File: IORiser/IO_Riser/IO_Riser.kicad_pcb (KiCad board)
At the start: 2 copper layers, 29.9 x 82.4 mm, 4 parts, among them J1 I/O Port, J2 I/O Port

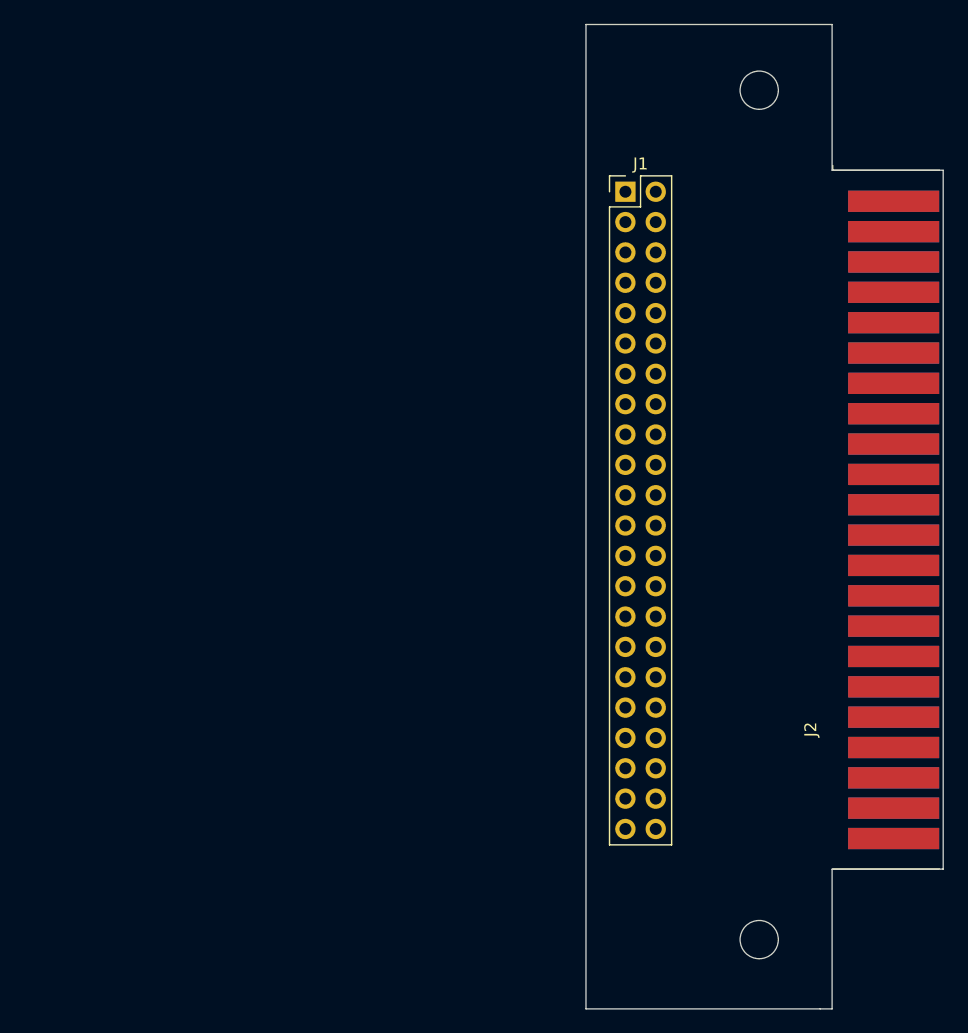
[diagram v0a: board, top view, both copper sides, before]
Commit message: PCB updates
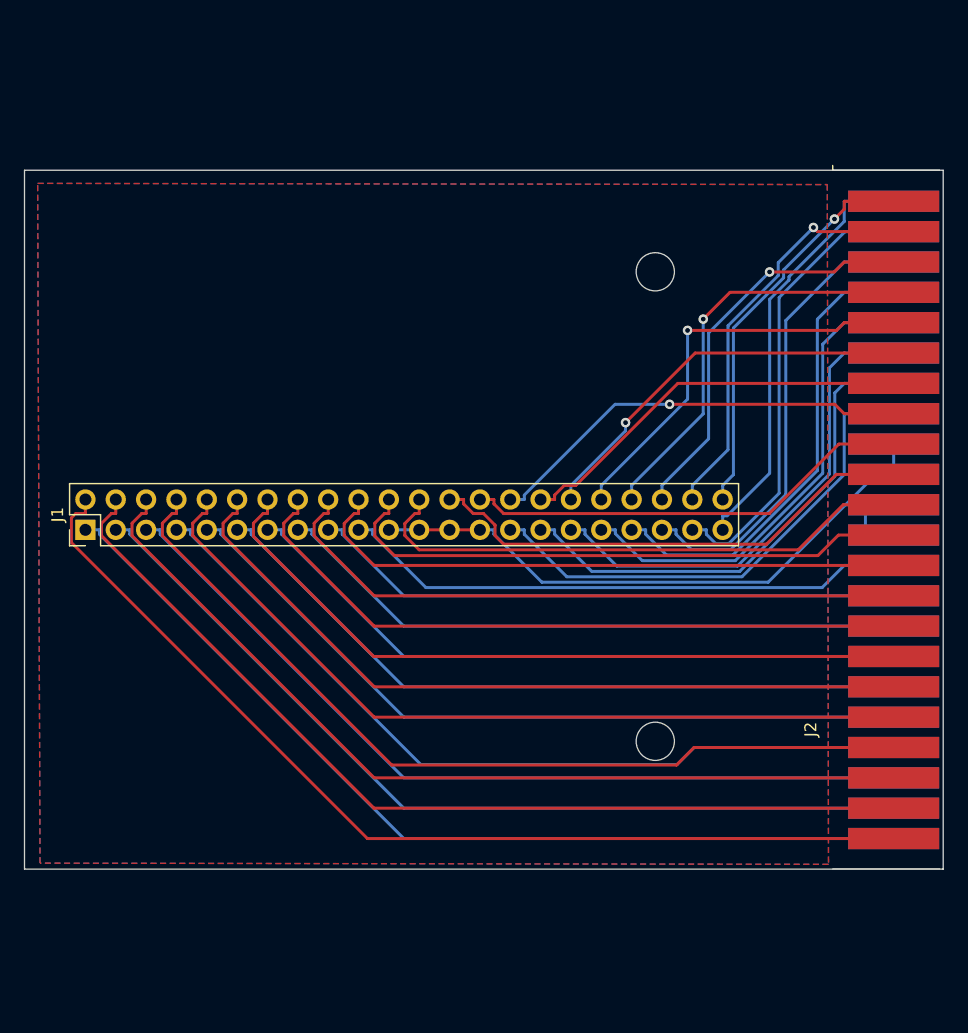
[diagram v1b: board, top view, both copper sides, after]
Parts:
- moved J1 53.3 mm to (97.8, 85.5), turned to 90 degrees
- moved H3 18.7 mm to (145.5, 103.2)
- moved H4 17.5 mm to (145.5, 63.9)
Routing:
- net SBE: track 0.00 -> 83.7 mm
- net ~{IO_EXT_INT}: track 0.00 -> 79.5 mm
- net +5V: track 0.00 -> 78.6 mm
- net IO_A10: track 0.00 -> 75.9 mm
- net ~{IO_RESET}: track 0.00 -> 75.0 mm
- net IO_A11: track 0.00 -> 73.5 mm
- net IO_A5: track 0.00 -> 71.4 mm
- net IO_A4: track 0.00 -> 69.0 mm
- net IO_A3: track 0.00 -> 68.7 mm
- net READY_~{HOLD}: track 0.00 -> 65.1 mm
- net IO_DBIN: track 0.00 -> 64.2 mm
- net IO_A8: track 0.00 -> 61.5 mm
- net IO_A12: track 0.00 -> 60.6 mm
- net GND: track 0.00 -> 59.6 mm
- net IO_A14: track 0.00 -> 57.9 mm
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- added copper zone on B.Cu, net GND
- added copper zone on F.Cu, net GND
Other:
- board size 29.9 x 82.4 mm -> 76.9 x 58.5 mm
